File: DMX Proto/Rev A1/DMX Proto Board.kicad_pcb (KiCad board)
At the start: 2 copper layers, 57 x 41 mm, 22 parts, among them J1 XLR5, J2 XLR5, J3 CONN_01X02_MALE, J4 CONN_01X02_MALE, J5 CONN_01X02_MALE, J6 CONN_01X02_MALE, T3 EXMACHINA-LOGO-NAME, U1 MAX481, U2 MAX481, U3 TCMT1600, U4 TCMT1600

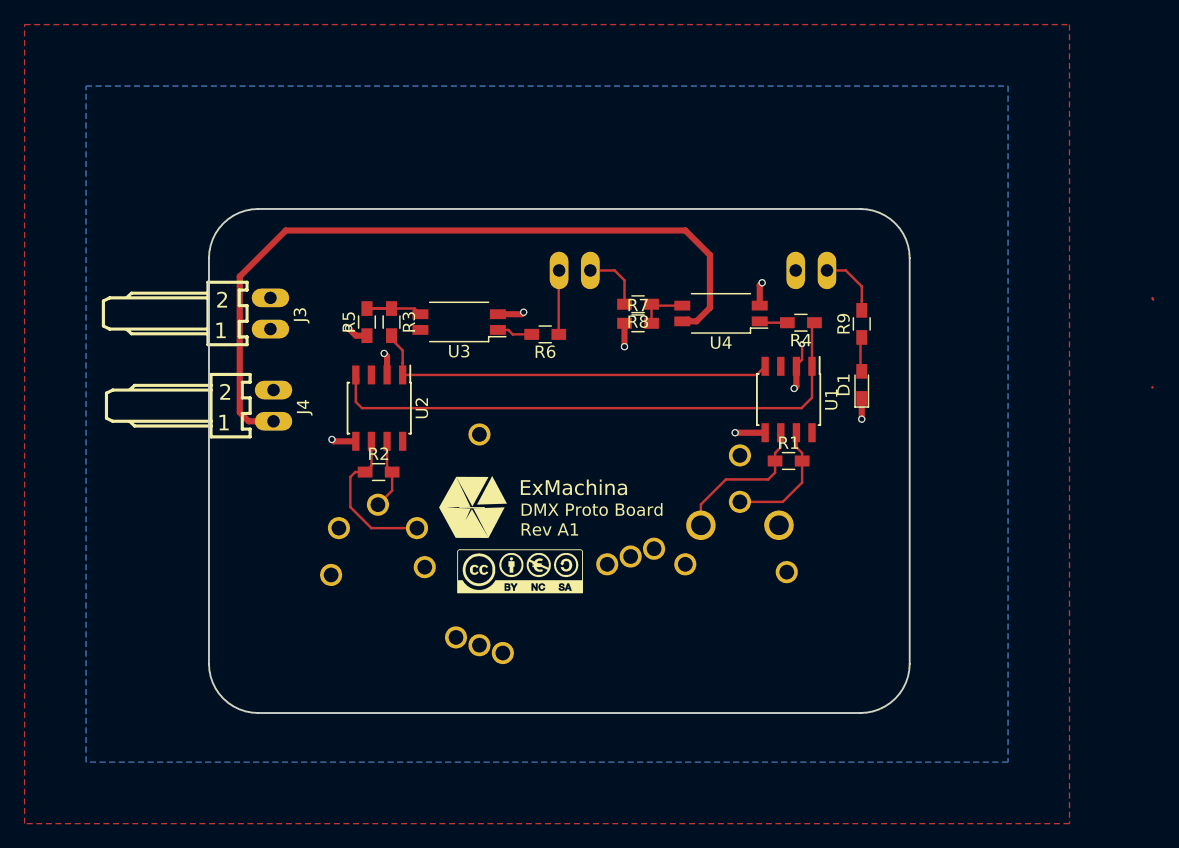
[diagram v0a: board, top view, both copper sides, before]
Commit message: Route the board and generate gerber
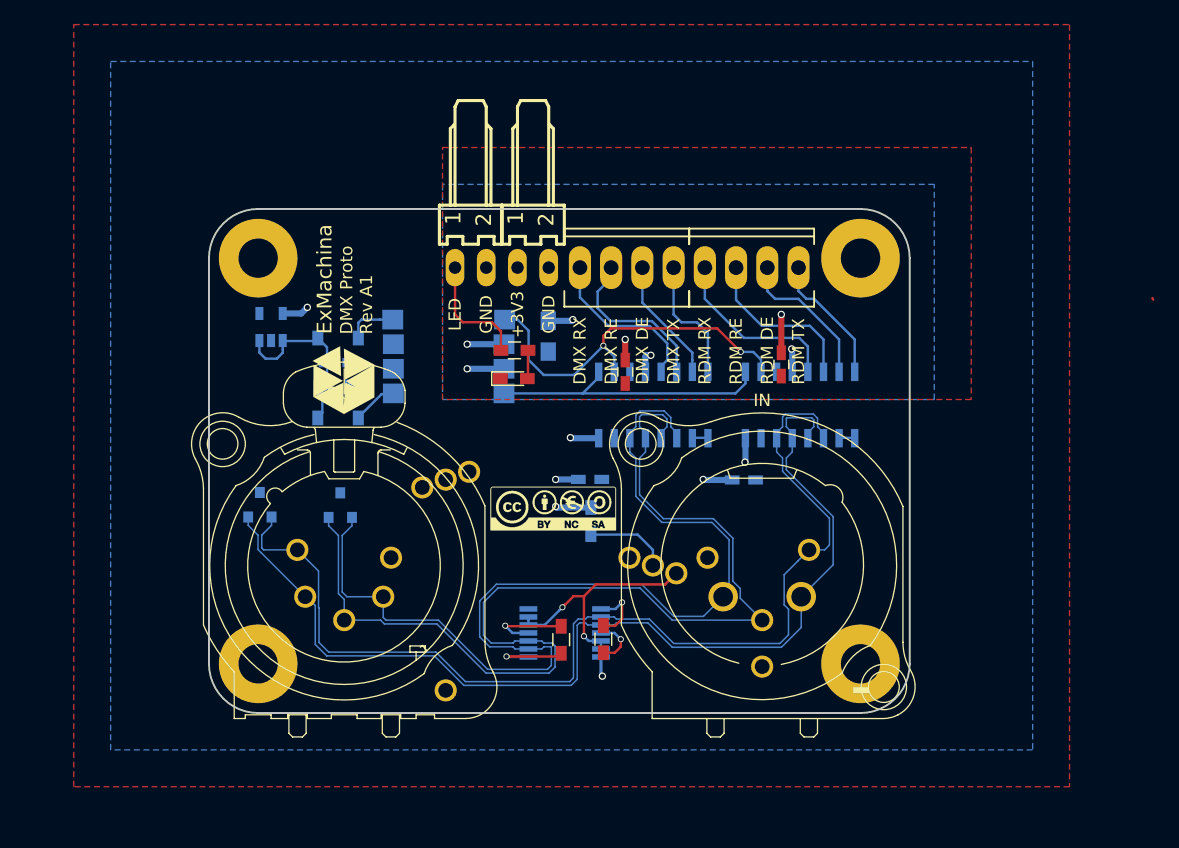
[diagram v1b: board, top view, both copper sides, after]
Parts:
- removed R4, R6, R8: 1K, Resistors_SMD:R_0603_HandSoldering
- removed R5, R7: 4K7, Resistors_SMD:R_0603_HandSoldering
- added C1: 100nF, Capacitors_SMD:C_0603_HandSoldering, B.Cu at (110.5, 72.5)
- added C2: 10uF, Capacitors_SMD:C_0805_HandSoldering, B.Cu at (110.5, 74.5)
- added C3: 100nF, Capacitors_SMD:C_0603_HandSoldering, B.Cu at (143.5, 82.0)
- added C4: 100nF, Capacitors_SMD:C_0603_HandSoldering, B.Cu at (131.0, 82.0)
- added C5: 100nF, Capacitors_SMD:C_0603_HandSoldering, F.Cu at (133.9, 73.2)
- added C6: 100nF, Capacitors_SMD:C_0603_HandSoldering, F.Cu at (146.6, 72.6)
- added C7: 10uF, 50V, Capacitors_SMD:C_0805_HandSoldering, B.Cu at (127.6, 70.3)
- added D2: 1N5819HW-7-F, Diodes_SMD:D_SOD-123, B.Cu at (110.5, 77.0)
- added D3: 1N5819HW-7-F, Diodes_SMD:D_SOD-123, B.Cu at (110.5, 70.5)
- added REF**: M3_Pad, Mounting_Holes:MountingHole_3.2mm_M3_Pad, F.Cu at (104.0, 64.0)
- added REF**: M3_Pad, Mounting_Holes:MountingHole_3.2mm_M3_Pad, F.Cu at (104.0, 97.0)
- added REF**: M3_Pad, Mounting_Holes:MountingHole_3.2mm_M3_Pad, F.Cu at (153.0, 64.0)
- added REF**: M3_Pad, Mounting_Holes:MountingHole_3.2mm_M3_Pad, F.Cu at (153.0, 97.0)
- added U5: PSM712, TO_SOT_Packages_SMD:SOT-23, B.Cu at (110.7, 84.1)
- added U6: PSM712, TO_SOT_Packages_SMD:SOT-23, B.Cu at (104.1, 84.1)
- added U7: MAX4751, Housings_SSOP:TSSOP-14_4.4x5mm_Pitch0.65mm, B.Cu at (128.9, 94.5)
- J1: value XLR5 -> NC5MAH; footprint Neutrix:NC5MAV-SW -> NC5MAV-SW; moved to F.Cu
- J2: value XLR5 -> NC5FAH; footprint Neutrix:NC5FAV-SW -> NC5FAV-SW; moved to F.Cu
- J3: value CONN_01X02_MALE -> 22-05-7048; footprint conn_Molex:7395-02 -> Sockets_MOLEX_KK-System:Socket_MOLEX-KK-RM2-54mm_Lock_4pin_straight
- J4: value CONN_01X02_MALE -> 22-05-7028
- J5: value CONN_01X02_MALE -> 22-05-7048; footprint conn_Molex:7395-02 -> Sockets_MOLEX_KK-System:Socket_MOLEX-KK-RM2-54mm_Lock_4pin_straight; moved to F.Cu
- J6: value CONN_01X02_MALE -> 22-05-7028; moved to F.Cu
- R1, R2: value 120 -> 120R
- R3: moved to B.Cu
- U1, U2: value MAX481 -> ISO35T; footprint Housings_SOIC:SOIC-8_3.9x4.9mm_Pitch1.27mm -> Housings_SOIC:SOIC-16_3.9x9.9mm_Pitch1.27mm; moved to B.Cu
- U3: value TCMT1600 -> TPS76333; footprint Housings_SSOP:SOP-4_4.4x2.8mm_Pitch1.27mm -> TO_SOT_Packages_SMD:SOT-23-5; moved to B.Cu
- U4: value TCMT1600 -> DA2303-AL; footprint Housings_SSOP:SOP-4_4.4x2.8mm_Pitch1.27mm -> CoilCraft:transformer-8-10x12.07; moved to B.Cu
- moved U2 34.2 mm to (148.1, 75.9)
- moved J3 29.2 mm to (134.0, 64.8), turned to 0 degrees
- moved R9 28.3 mm to (124.8, 71.5), turned to 180 degrees
- moved D1 28.3 mm to (124.8, 73.8), turned to 0 degrees
- moved J6 27.7 mm to (121.3, 64.8), turned to 180 degrees
- moved J4 23.9 mm to (126.4, 64.8), turned to 180 degrees
- moved R1 23.5 mm to (128.7, 95.0), turned to 90 degrees
- moved R3 22.9 mm to (131.1, 85.4)
- moved R2 22.8 mm to (132.1, 95.0), turned to 270 degrees
- moved U4 22.4 mm to (119.5, 72.0)
- moved U3 15.3 mm to (105.0, 69.6), turned to 90 degrees
- moved T3 14.6 mm to (111.0, 74.0), turned to 90 degrees
- moved J5 14.4 mm to (144.1, 64.8)
- moved U1 11.0 mm to (136.1, 75.9)
- moved S? 5.77 mm to (128.0, 84.4)
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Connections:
- D1 pad 1: GND -> GNDA
- J1 pad 2: DMX_IN_A -> DMX+
- J1 pad 3: DMX_IN_B -> DMX-
- J1 pad 4: Net-(J1-Pad4) -> RDM-
- J1 pad 5: Net-(J1-Pad5) -> RDM+
- J1 pad N: (no net) -> Net-(J1-PadN)
- J1 pad NC: (no net) -> Net-(J1-PadNC)
- J2 pad 2: DMX_OUT_A -> DMX+
- J2 pad 3: DMX_OUT_B -> DMX-
- J2 pad 4: Net-(J2-Pad4) -> RDM-
- J2 pad 5: Net-(J2-Pad5) -> RDM+
- J3 pad 1: +5V -> DMX_MCU_RX
- J3 pad 2: GND -> DMX_MCU_RE
- J4 pad 1: +3V3 -> +3.3VA
- J4 pad 2: GND -> GNDA
- J5 pad 1: DMX_MCU_RX -> RDM_MCU_RX
- J5 pad 2: DMX_MCU_TX -> RDM_MCU_RE
- J6 pad 2: GND -> GNDA
- R1 pad 1: DMX_IN_A -> Net-(R1-Pad1)
- R1 pad 2: DMX_IN_B -> Net-(R1-Pad2)
- R2 pad 1: DMX_OUT_A -> Net-(R2-Pad1)
- R2 pad 2: DMX_OUT_B -> Net-(R2-Pad2)
- R3 pad 1: Net-(R3-Pad1) -> +3V3
- R3 pad 2: DMX_TX -> Net-(J1-PadN)
- U1 pad 1: DMX_RX -> Transformer_Driver_1
- U1 pad 2: GND -> Transformer_Driver_2
- U1 pad 3: +5V -> GNDA
- U1 pad 4: DMX_TX -> +3.3VA
- U1 pad 5: GND -> DMX_MCU_RX
- U1 pad 6: DMX_IN_A -> DMX_MCU_RE
- U1 pad 7: DMX_IN_B -> DMX_MCU_DE
- U1 pad 8: +5V -> DMX_MCU_TX
- U2 pad 1: DMX_TX -> Transformer_Driver_1
- U2 pad 2: GND -> Transformer_Driver_2
- U2 pad 3: +5V -> GNDA
- U2 pad 4: DMX_RX -> +3.3VA
- U2 pad 5: GND -> RDM_MCU_RX
- U2 pad 6: DMX_OUT_A -> RDM_MCU_RE
- U2 pad 7: DMX_OUT_B -> RDM_MCU_DE
- U2 pad 8: +5V -> RDM_MCU_TX
- U3 pad 1: Net-(R6-Pad2) -> Net-(C1-Pad1)
- U3 pad 3: Net-(R3-Pad1) -> Net-(C1-Pad1)
- U3 pad 4: +5V -> (no net)
- U4 pad 1: Net-(R4-Pad2) -> Transformer_Driver_2
- U4 pad 2: GND -> +3.3VA
- U4 pad 3: Net-(R7-Pad2) -> +3.3VA
- U4 pad 4: +3V3 -> Transformer_Driver_1
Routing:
- net DMX-: track 0.00 -> 90.6 mm
- net RDM+: track 0.00 -> 87.0 mm
- net DMX+: track 0.00 -> 86.1 mm
- net RDM-: track 0.00 -> 84.6 mm
- net +3V3: track 64.1 -> 15.3 mm, vias 0 -> 7
- net DMX_RX: track 46.5 -> 0.00 mm
- net DMX_TX: track 33.5 -> 0.00 mm
- net Transformer_Driver_2: track 0.00 -> 30.7 mm, vias 0 -> 2
- net Transformer_Driver_1: track 0.00 -> 23.2 mm
- net Net-(J1-PadNC): track 0.00 -> 19.8 mm, vias 0 -> 2
- net +3.3VA: track 0.00 -> 16.4 mm, vias 0 -> 7
- net GND: track 19.8 -> 4.16 mm, vias 10 -> 0
- net Net-(C1-Pad1): track 0.00 -> 14.7 mm
- net RDM_MCU_RX: track 0.00 -> 14.6 mm
- net RDM_MCU_RE: track 0.00 -> 13.7 mm
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- added copper zone on In1.Cu, net +3.3VA
- added copper zone on In1.Cu, net +3V3
- added copper zone on F.Cu, net GND
- added copper zone on In2.Cu, net GND
- added copper zone on B.Cu, net GNDA
- added copper zone on F.Cu, net GNDA
- added copper zone on In2.Cu, net GNDA
- removed copper zone on F.Cu, net +5V
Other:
- copper layers 2 -> 4
- net class Differential added: clearance 0.125, trace_width 0.125, via_dia 0.5, via_drill 0.35
- rule trace_min: 0.2 -> 0.125
- board text added: "+3V3"
- board text added: "DMX DE"
- board text added: "DMX Proto Rev A1"
- board text added: "DMX RE"
- board text added: "DMX RX"
- board text added: "DMX TX"
- board text added: "GND"
- board text added: "IN"
- board text added: "LED"
- board text added: "OUT"
- board text added: "RDM DE"
- board text added: "RDM RE"
- board text added: "RDM RX"
- board text added: "RDM TX"
- board text removed: "DMX Proto Board Rev A1"
